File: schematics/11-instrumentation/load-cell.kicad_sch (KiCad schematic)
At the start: 9 parts, among them J9 HX711, U10 PCA9306

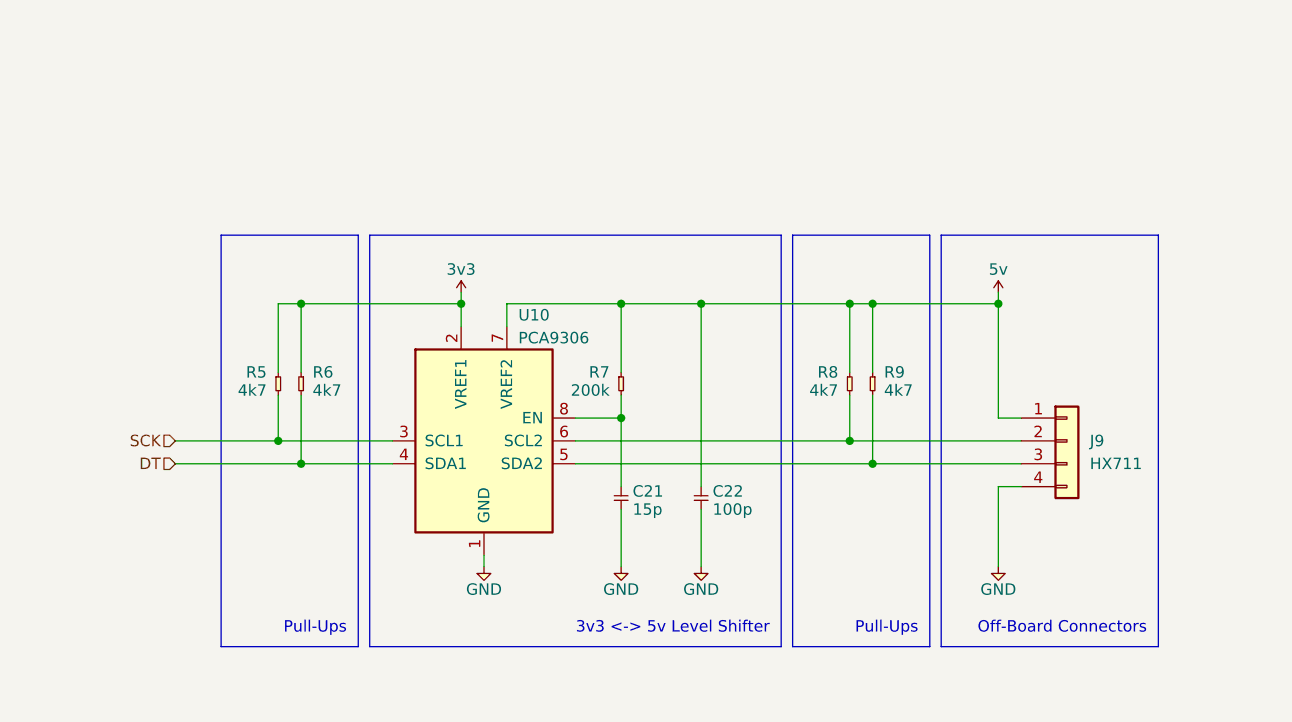
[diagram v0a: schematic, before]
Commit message: Added stuff
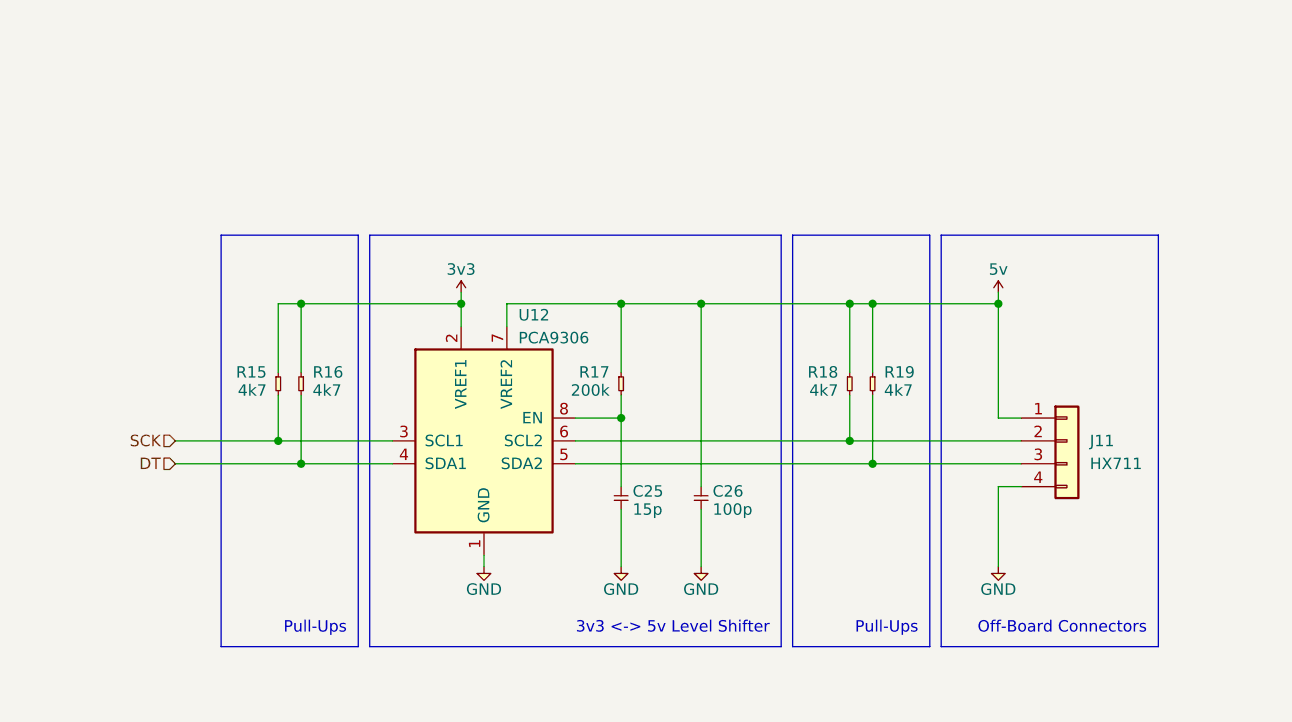
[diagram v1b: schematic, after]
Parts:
- renumbered C21 to C25, C22 to C26, J9 to J11, R5 to R15, R6 to R16, R7 to R17, R8 to R18, R9 to R19, U10 to U12
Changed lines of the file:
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@@
   (symbol (lib_id "royale:C") (at 144.78 99.06 270)
     (in_bom yes) (on_board yes)
-    (property "Reference" "C21" (id 0) (at 146.05 100.33 90)
+    (property "Reference" "C25" (id 0) (at 146.05 100.33 90)
       (effects (font (size 1.27 1.27)) (justify left bottom))
     )
@@
   (symbol (lib_id "cusf-kicad:GND") (at 144.78 107.95 0)
     (in_bom yes) (on_board yes)
-    (property "Reference" "#PWR032" (id 0) (at 141.478 106.934 0)
+    (property "Reference" "#PWR044" (id 0) (at 141.478 106.934 0)
       (effects (font (size 1.27 1.27)) (justify left) hide)
     )
@@
   (symbol (lib_id "royale:R") (at 144.78 86.36 90) (mirror x)
     (in_bom yes) (on_board yes)
-    (property "Reference" "R7" (id 0) (at 143.51 86.36 90)
+    (property "Reference" "R17" (id 0) (at 143.51 86.36 90)
       (effects (font (size 1.27 1.27)) (justify left))
     )
@@
   (symbol (lib_id "royale:3v3") (at 127 77.47 0)
     (in_bom yes) (on_board yes)
-    (property "Reference" "#PWR030" (id 0) (at 127 74.676 0)
+    (property "Reference" "#PWR042" (id 0) (at 127 74.676 0)
       (effects (font (size 1.27 1.27)) (justify left) hide)
     )
@@
   (symbol (lib_id "cusf-kicad:GND") (at 129.54 107.95 0)
     (in_bom yes) (on_board yes)
-    (property "Reference" "#PWR031" (id 0) (at 126.238 106.934 0)
+    (property "Reference" "#PWR043" (id 0) (at 126.238 106.934 0)
       (effects (font (size 1.27 1.27)) (justify left) hide)
     )
@@
   (symbol (lib_id "royale:PCA9306") (at 129.54 93.98 0)
     (in_bom yes) (on_board yes)
-    (property "Reference" "U10" (id 0) (at 133.35 80.01 0)
+    (property "Reference" "U12" (id 0) (at 133.35 80.01 0)
       (effects (font (size 1.27 1.27)) (justify left))
     )
@@
   (symbol (lib_id "royale:5v") (at 186.69 77.47 0)
     (in_bom yes) (on_board yes)
-    (property "Reference" "#PWR034" (id 0) (at 186.69 74.676 0)
+    (property "Reference" "#PWR046" (id 0) (at 186.69 74.676 0)
       (effects (font (size 1.27 1.27)) (justify left) hide)
     )
@@
   (symbol (lib_id "cusf-kicad:GND") (at 186.69 107.95 0)
     (in_bom yes) (on_board yes)
-    (property "Reference" "#PWR035" (id 0) (at 183.388 106.934 0)
+    (property "Reference" "#PWR047" (id 0) (at 183.388 106.934 0)
       (effects (font (size 1.27 1.27)) (justify left) hide)
     )
@@
   (symbol (lib_id "royale:Conn_01x04") (at 194.31 93.98 0)
     (in_bom yes) (on_board yes)
-    (property "Reference" "J9" (id 0) (at 196.85 93.98 0)
+    (property "Reference" "J11" (id 0) (at 196.85 93.98 0)
       (effects (font (size 1.27 1.27)) (justify left))
     )
@@
   (symbol (lib_id "royale:R") (at 172.72 86.36 270)
     (in_bom yes) (on_board yes)
-    (property "Reference" "R9" (id 0) (at 173.99 86.36 90)
+    (property "Reference" "R19" (id 0) (at 173.99 86.36 90)
       (effects (font (size 1.27 1.27)) (justify left))
     )
@@
   (symbol (lib_id "royale:R") (at 170.18 86.36 90) (mirror x)
     (in_bom yes) (on_board yes)
-    (property "Reference" "R8" (id 0) (at 168.91 86.36 90)
+    (property "Reference" "R18" (id 0) (at 168.91 86.36 90)
       (effects (font (size 1.27 1.27)) (justify left))
     )
@@
   (symbol (lib_id "royale:C") (at 153.67 99.06 270)
     (in_bom yes) (on_board yes)
-    (property "Reference" "C22" (id 0) (at 154.94 100.33 90)
+    (property "Reference" "C26" (id 0) (at 154.94 100.33 90)
       (effects (font (size 1.27 1.27)) (justify left bottom))
     )
@@
   (symbol (lib_id "cusf-kicad:GND") (at 153.67 107.95 0)
     (in_bom yes) (on_board yes)
-    (property "Reference" "#PWR033" (id 0) (at 150.368 106.934 0)
+    (property "Reference" "#PWR045" (id 0) (at 150.368 106.934 0)
       (effects (font (size 1.27 1.27)) (justify left) hide)
     )
@@
   (symbol (lib_id "royale:R") (at 109.22 86.36 270)
     (in_bom yes) (on_board yes)
-    (property "Reference" "R6" (id 0) (at 110.49 86.36 90)
+    (property "Reference" "R16" (id 0) (at 110.49 86.36 90)
       (effects (font (size 1.27 1.27)) (justify left))
     )
@@
   (symbol (lib_id "royale:R") (at 106.68 86.36 90) (mirror x)
     (in_bom yes) (on_board yes)
-    (property "Reference" "R5" (id 0) (at 105.41 86.36 90)
-      (effects (font (size 1.27 1.27)) (justify left))
-    )
+    (property "Reference" "R15" (id 0) (at 105.41 86.36 90)
+      (effects (font (size 1.27 1.27)) (justify left))
+    )

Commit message: Revert instrumentation to master
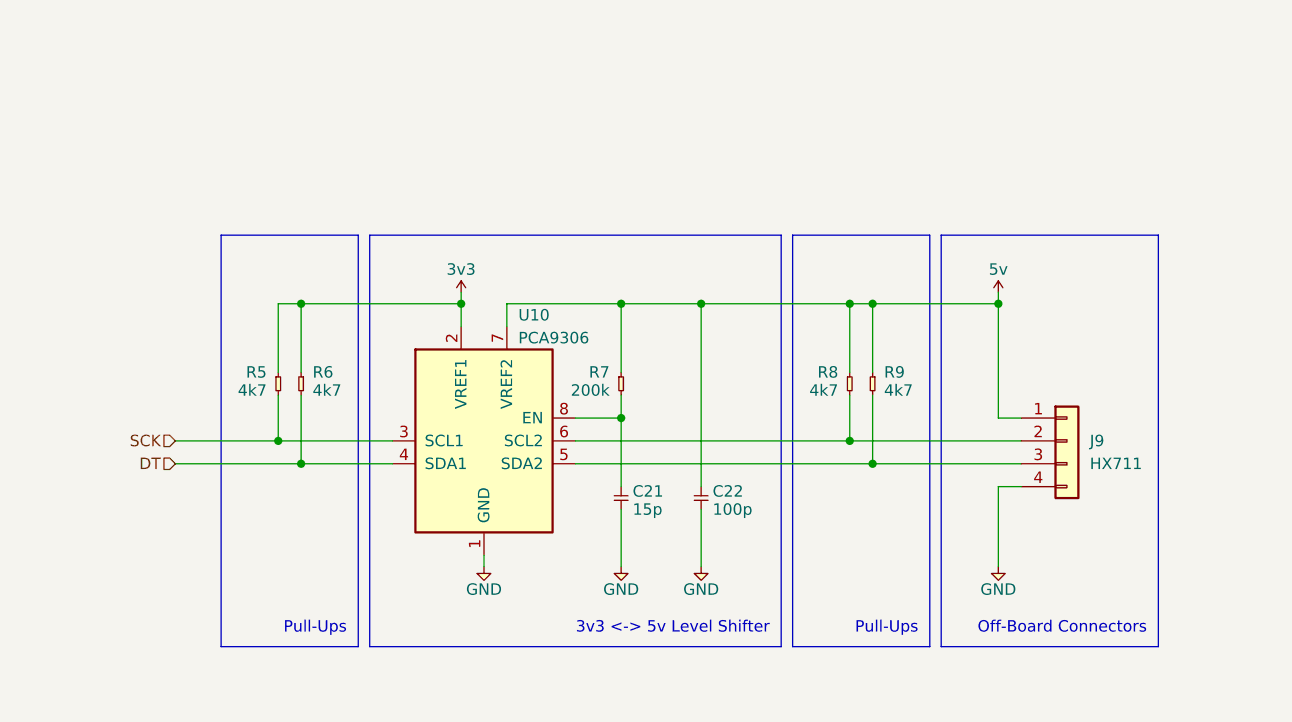
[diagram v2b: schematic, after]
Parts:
- renumbered C25 to C21, C26 to C22, J11 to J9, R15 to R5, R16 to R6, R17 to R7, R18 to R8, R19 to R9, U12 to U10
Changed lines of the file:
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@@
   (symbol (lib_id "royale:C") (at 144.78 99.06 270)
     (in_bom yes) (on_board yes)
-    (property "Reference" "C25" (id 0) (at 146.05 100.33 90)
+    (property "Reference" "C21" (id 0) (at 146.05 100.33 90)
       (effects (font (size 1.27 1.27)) (justify left bottom))
     )
@@
   (symbol (lib_id "cusf-kicad:GND") (at 144.78 107.95 0)
     (in_bom yes) (on_board yes)
-    (property "Reference" "#PWR044" (id 0) (at 141.478 106.934 0)
+    (property "Reference" "#PWR032" (id 0) (at 141.478 106.934 0)
       (effects (font (size 1.27 1.27)) (justify left) hide)
     )
@@
   (symbol (lib_id "royale:R") (at 144.78 86.36 90) (mirror x)
     (in_bom yes) (on_board yes)
-    (property "Reference" "R17" (id 0) (at 143.51 86.36 90)
+    (property "Reference" "R7" (id 0) (at 143.51 86.36 90)
       (effects (font (size 1.27 1.27)) (justify left))
     )
@@
   (symbol (lib_id "royale:3v3") (at 127 77.47 0)
     (in_bom yes) (on_board yes)
-    (property "Reference" "#PWR042" (id 0) (at 127 74.676 0)
+    (property "Reference" "#PWR030" (id 0) (at 127 74.676 0)
       (effects (font (size 1.27 1.27)) (justify left) hide)
     )
@@
   (symbol (lib_id "cusf-kicad:GND") (at 129.54 107.95 0)
     (in_bom yes) (on_board yes)
-    (property "Reference" "#PWR043" (id 0) (at 126.238 106.934 0)
+    (property "Reference" "#PWR031" (id 0) (at 126.238 106.934 0)
       (effects (font (size 1.27 1.27)) (justify left) hide)
     )
@@
   (symbol (lib_id "royale:PCA9306") (at 129.54 93.98 0)
     (in_bom yes) (on_board yes)
-    (property "Reference" "U12" (id 0) (at 133.35 80.01 0)
+    (property "Reference" "U10" (id 0) (at 133.35 80.01 0)
       (effects (font (size 1.27 1.27)) (justify left))
     )
@@
   (symbol (lib_id "royale:5v") (at 186.69 77.47 0)
     (in_bom yes) (on_board yes)
-    (property "Reference" "#PWR046" (id 0) (at 186.69 74.676 0)
+    (property "Reference" "#PWR034" (id 0) (at 186.69 74.676 0)
       (effects (font (size 1.27 1.27)) (justify left) hide)
     )
@@
   (symbol (lib_id "cusf-kicad:GND") (at 186.69 107.95 0)
     (in_bom yes) (on_board yes)
-    (property "Reference" "#PWR047" (id 0) (at 183.388 106.934 0)
+    (property "Reference" "#PWR035" (id 0) (at 183.388 106.934 0)
       (effects (font (size 1.27 1.27)) (justify left) hide)
     )
@@
   (symbol (lib_id "royale:Conn_01x04") (at 194.31 93.98 0)
     (in_bom yes) (on_board yes)
-    (property "Reference" "J11" (id 0) (at 196.85 93.98 0)
+    (property "Reference" "J9" (id 0) (at 196.85 93.98 0)
       (effects (font (size 1.27 1.27)) (justify left))
     )
@@
   (symbol (lib_id "royale:R") (at 172.72 86.36 270)
     (in_bom yes) (on_board yes)
-    (property "Reference" "R19" (id 0) (at 173.99 86.36 90)
+    (property "Reference" "R9" (id 0) (at 173.99 86.36 90)
       (effects (font (size 1.27 1.27)) (justify left))
     )
@@
   (symbol (lib_id "royale:R") (at 170.18 86.36 90) (mirror x)
     (in_bom yes) (on_board yes)
-    (property "Reference" "R18" (id 0) (at 168.91 86.36 90)
+    (property "Reference" "R8" (id 0) (at 168.91 86.36 90)
       (effects (font (size 1.27 1.27)) (justify left))
     )
@@
   (symbol (lib_id "royale:C") (at 153.67 99.06 270)
     (in_bom yes) (on_board yes)
-    (property "Reference" "C26" (id 0) (at 154.94 100.33 90)
+    (property "Reference" "C22" (id 0) (at 154.94 100.33 90)
       (effects (font (size 1.27 1.27)) (justify left bottom))
     )
@@
   (symbol (lib_id "cusf-kicad:GND") (at 153.67 107.95 0)
     (in_bom yes) (on_board yes)
-    (property "Reference" "#PWR045" (id 0) (at 150.368 106.934 0)
+    (property "Reference" "#PWR033" (id 0) (at 150.368 106.934 0)
       (effects (font (size 1.27 1.27)) (justify left) hide)
     )
@@
   (symbol (lib_id "royale:R") (at 109.22 86.36 270)
     (in_bom yes) (on_board yes)
-    (property "Reference" "R16" (id 0) (at 110.49 86.36 90)
+    (property "Reference" "R6" (id 0) (at 110.49 86.36 90)
       (effects (font (size 1.27 1.27)) (justify left))
     )
@@
   (symbol (lib_id "royale:R") (at 106.68 86.36 90) (mirror x)
     (in_bom yes) (on_board yes)
-    (property "Reference" "R15" (id 0) (at 105.41 86.36 90)
-      (effects (font (size 1.27 1.27)) (justify left))
-    )
+    (property "Reference" "R5" (id 0) (at 105.41 86.36 90)
+      (effects (font (size 1.27 1.27)) (justify left))
+    )

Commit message: load cell
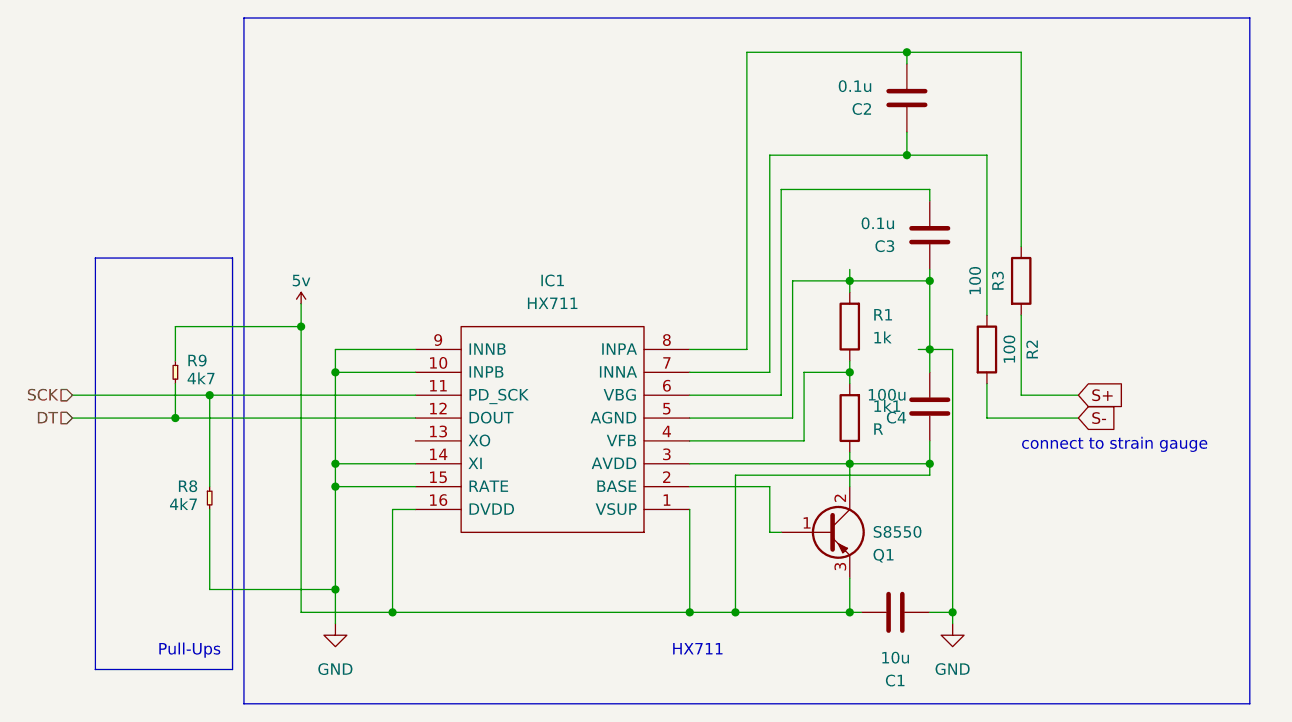
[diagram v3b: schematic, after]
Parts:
- removed C21: 15p, royale:C_0402_1005Metric_Pad0.74x0.62mm_HandSolder, symbol royale:C
- removed C22: 100p, royale:C_0402_1005Metric_Pad0.74x0.62mm_HandSolder, symbol royale:C
- removed J9: HX711, symbol royale:Conn_01x04
- removed R5, R6: 4k7, symbol royale:R
- removed R7: 200k, royale:R_0402_1005Metric_Pad0.72x0.64mm_HandSolder, symbol royale:R
- removed U10: PCA9306, symbol royale:PCA9306
- added 1k1: R, symbol Device:R
- added C1: 10u, symbol Device:C
- added C2, C3: 0.1u, symbol Device:C
- added C4: 100u, symbol Device:C
- added IC1: HX711, SOIC127P600X160-16N, symbol HX711:HX711
- added Q1: S8550, symbol Device:Q_PNP_BCE
- added R1: 1k, symbol Device:R
- added R2, R3: 100, symbol Device:R
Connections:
- net 1v8: now also 1k1.1, C1.2, C4.1, IC1.1 (VSUP), IC1.16 (DVDD), IC1.3 (AVDD), Q1.2 (C), Q1.3 (E); no longer R8.1
- net DT: now also R9.2, IC1.12 (DOUT)
- net GND: now also R8.2, C1.1, C3.1, C4.2, IC1.10 (INPB), IC1.14 (XI), IC1.15 (RATE), IC1.5 (AGND), IC1.9 (INNB), R1.2
- net SCK: now also R8.1, IC1.11 (PD_SCK)
- new net: C3.2, IC1.6 (VBG)
- new net: C2.2, IC1.8 (INPA), R3.1
- new net: IC1.2 (BASE), Q1.1 (B)
- new net: 1k1.2, IC1.4 (VFB), R1.1
- new net: C2.1, IC1.7 (INNA), R2.1
- new net S+: R3.2
- new net S-: R2.2
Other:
- note added: "HX711"
- note added: "connect to strain gauge"
- note removed: "3v3 <-> 5v Level Shifter"
- note removed: "Off-Board Connectors"
- moved on the sheet: R8, R9
